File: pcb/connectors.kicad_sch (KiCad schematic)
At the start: 5 parts, among them J20 DTM1312PA12PBR008, U8 EEC-325X4B

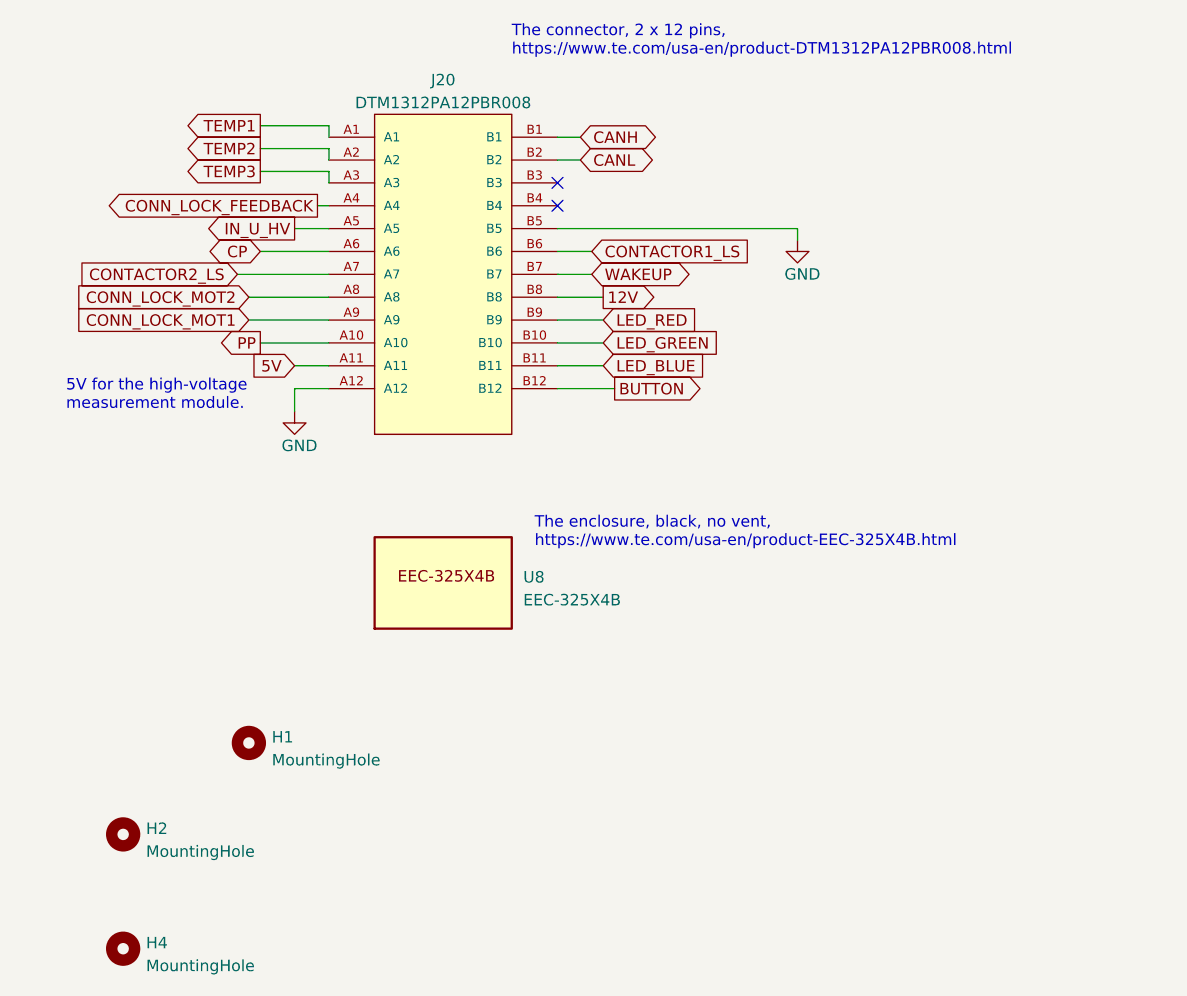
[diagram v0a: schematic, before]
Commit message: Re-assigned pins to be able to make one loom to the charge port and one to the car
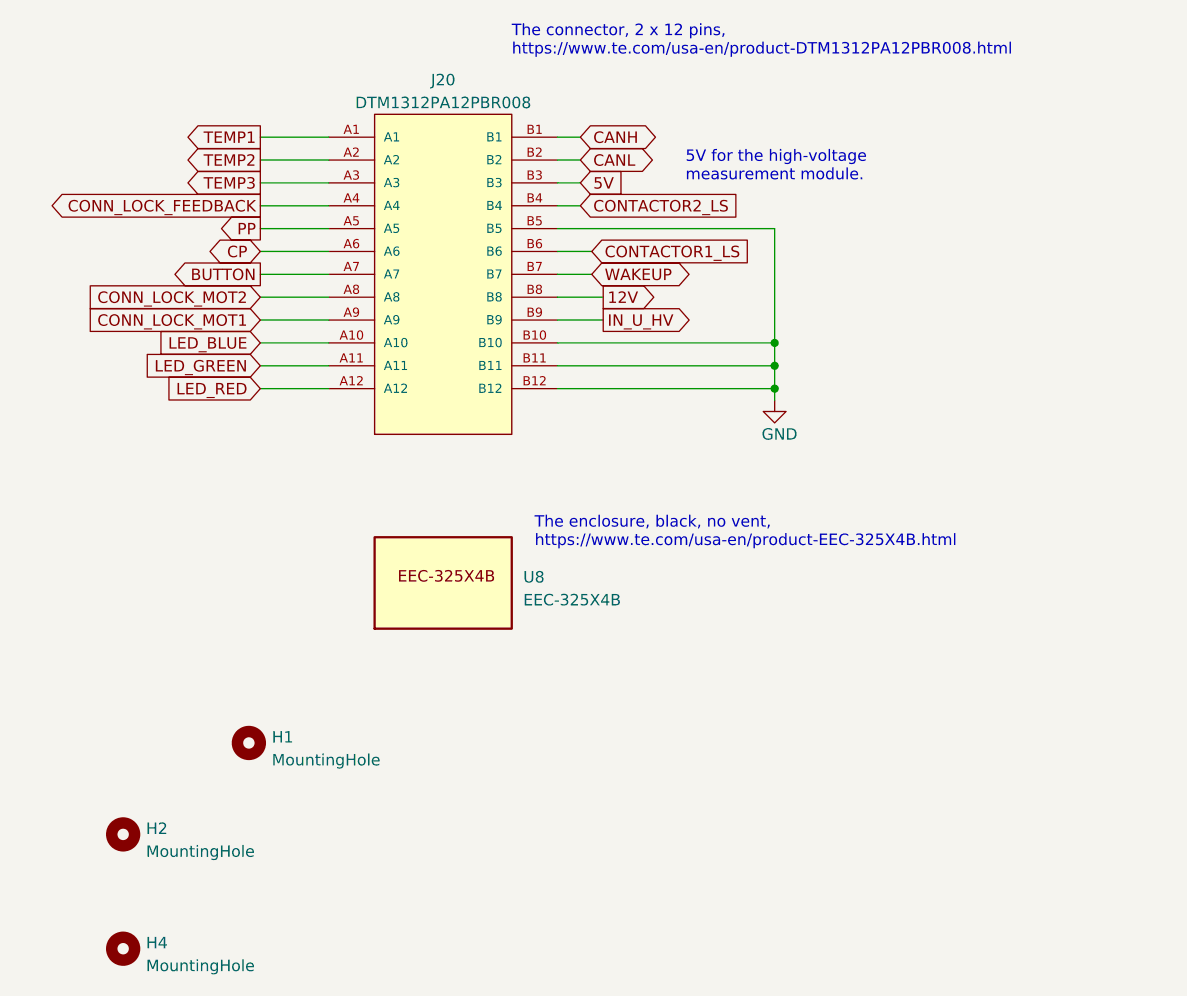
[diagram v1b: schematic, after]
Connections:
- net 5V: now also J20.B3; no longer J20.A11
- net BUTTON: now also J20.A7; no longer J20.B12
- net CONTACTOR2_LS: now also J20.B4; no longer J20.A7
- net GND: now also J20.B10, J20.B11, J20.B12; no longer J20.A12
- net IN_U_HV: now also J20.B9; no longer J20.A5
- net LED_BLUE: now also J20.A10; no longer J20.B11
- net LED_GREEN: now also J20.A11; no longer J20.B10
- net LED_RED: now also J20.A12; no longer J20.B9
- net PP: now also J20.A5; no longer J20.A10
- no-connect marks 2 -> 0

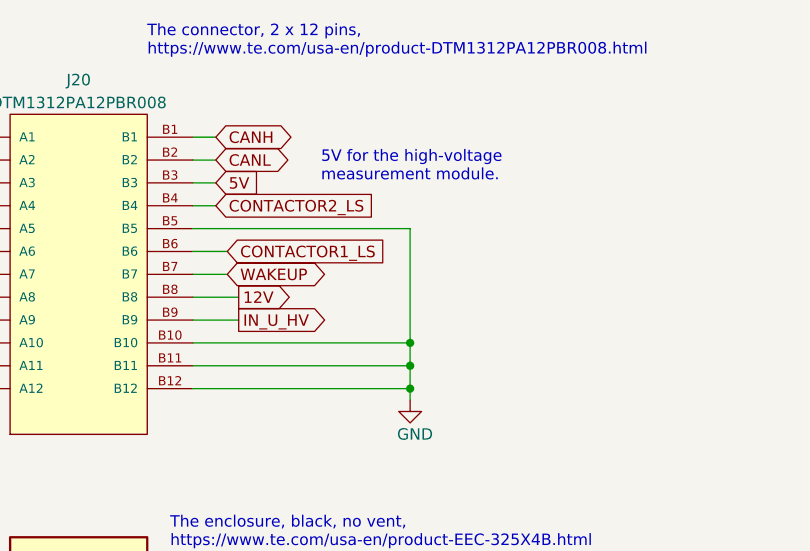
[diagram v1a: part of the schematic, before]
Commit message: More re-assignment
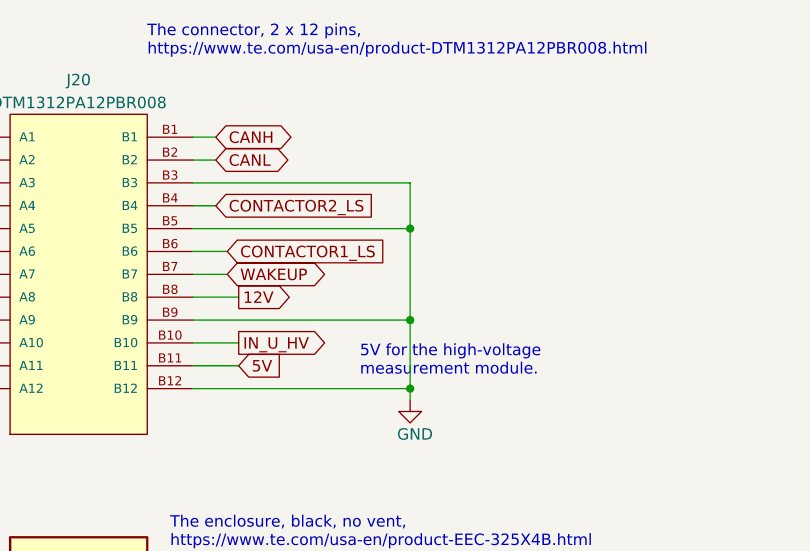
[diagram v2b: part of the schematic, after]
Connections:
- net 5V: now also J20.B11; no longer J20.B3
- net GND: now also J20.B3, J20.B9; no longer J20.B10, J20.B11
- net IN_U_HV: now also J20.B10; no longer J20.B9
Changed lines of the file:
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@@
 	(paper "A4")
 	(junction
-		(at 102.87 67.31)
+		(at 102.87 64.77)
+		(diameter 0)
+		(color 0 0 0 0)
+	)
+	(junction
+		(at 102.87 54.61)
 		(diameter 0)
 		(color 0 0 0 0)
@@
 		(color 0 0 0 0)
 	)
-	(junction
-		(at 102.87 69.85)
-		(diameter 0)
-		(color 0 0 0 0)
-	)
 	(wire
 		(pts
@@
 	(wire
 		(pts
-			(xy 102.87 72.39) (xy 102.87 69.85)
+			(xy 102.87 54.61) (xy 102.87 64.77)
 		)
 		(stroke
@@
 	(wire
 		(pts
+			(xy 78.74 67.31) (xy 83.82 67.31)
+		)
+		(stroke
+			(width 0)
+			(type default)
+		)
+	)
+	(wire
+		(pts
 			(xy 78.74 52.07) (xy 81.28 52.07)
 		)
@@
 	(wire
 		(pts
-			(xy 78.74 67.31) (xy 102.87 67.31)
+			(xy 78.74 49.53) (xy 102.87 49.53)
 		)
 		(stroke
@@
 	(wire
 		(pts
-			(xy 78.74 64.77) (xy 83.82 64.77)
+			(xy 78.74 64.77) (xy 102.87 64.77)
 		)
 		(stroke
@@
 	(wire
 		(pts
-			(xy 102.87 54.61) (xy 102.87 67.31)
-		)
-		(stroke
-			(width 0)
-			(type default)
-		)
-	)
-	(wire
-		(pts
 			(xy 45.72 54.61) (xy 53.34 54.61)
 		)
@@
 	(wire
 		(pts
-			(xy 102.87 69.85) (xy 102.87 67.31)
+			(xy 102.87 49.53) (xy 102.87 54.61)
+		)
+		(stroke
+			(width 0)
+			(type default)
+		)
+	)
+	(wire
+		(pts
+			(xy 102.87 64.77) (xy 102.87 72.39)
 		)
 		(stroke
@@
 	(wire
 		(pts
-			(xy 78.74 69.85) (xy 102.87 69.85)
-		)
-		(stroke
-			(width 0)
-			(type default)
-		)
-	)
-	(wire
-		(pts
 			(xy 78.74 46.99) (xy 81.28 46.99)
 		)
@@
 	(wire
 		(pts
+			(xy 78.74 69.85) (xy 83.82 69.85)
+		)
+		(stroke
+			(width 0)
+			(type default)
+		)
+	)
+	(wire
+		(pts
 			(xy 45.72 44.45) (xy 53.34 44.45)
-		)
-		(stroke
-			(width 0)
-			(type default)
-		)
-	)
-	(wire
-		(pts
-			(xy 78.74 49.53) (xy 81.28 49.53)
 		)
 		(stroke
@@
 	(text "5V for the high-voltage\nmeasurement module."
 		(exclude_from_sim no)
-		(at 92.964 49.53 0)
+		(at 97.282 71.12 0)
 		(effects
 			(font
@@
 	(global_label "5V"
 		(shape input)
-		(at 81.28 49.53 0)
+		(at 83.82 69.85 0)
 		(fields_autoplaced yes)
 		(effects
@@
 		)
 		(property "Intersheetrefs" "${INTERSHEET_REFS}"
-			(at 86.5633 49.53 0)
+			(at 89.1033 69.85 0)
 			(effects
 				(font
@@
 	(global_label "IN_U_HV"
 		(shape output)
-		(at 83.82 64.77 0)
+		(at 83.82 67.31 0)
 		(fields_autoplaced yes)
 		(effects
@@
 		)
 		(property "Intersheetrefs" "${INTERSHEET_REFS}"
-			(at 94.4253 64.77 0)
-			(effects
-				(font
+			(at 94.4253 67.31 0)
+			(effects
+				(font
